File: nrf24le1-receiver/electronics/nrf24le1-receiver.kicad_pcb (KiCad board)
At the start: 2 copper layers, 19 x 25 mm, 20 parts, among them K1 CONN_3, K2 CONN_3, K3 CONN_3, K4 CONN_3, P1 CONN_1, P2 CONN_1, P3 CONN_1, SW1 BIND, U1 MCP1703, U2 NRF24LE1-MODULE-15X21

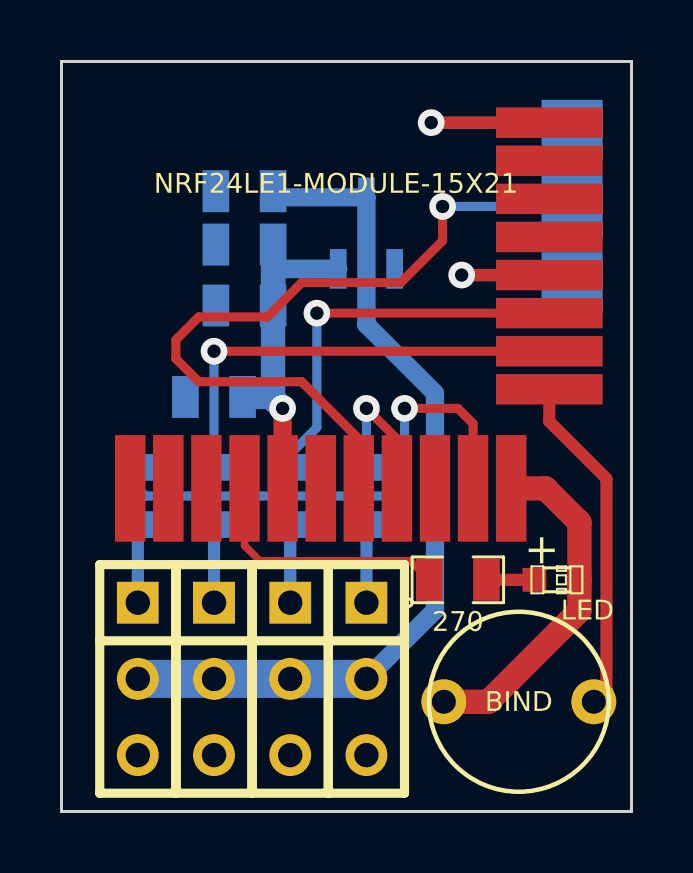
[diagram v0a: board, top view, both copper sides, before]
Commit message: Add Gerber for revision 2 PCB
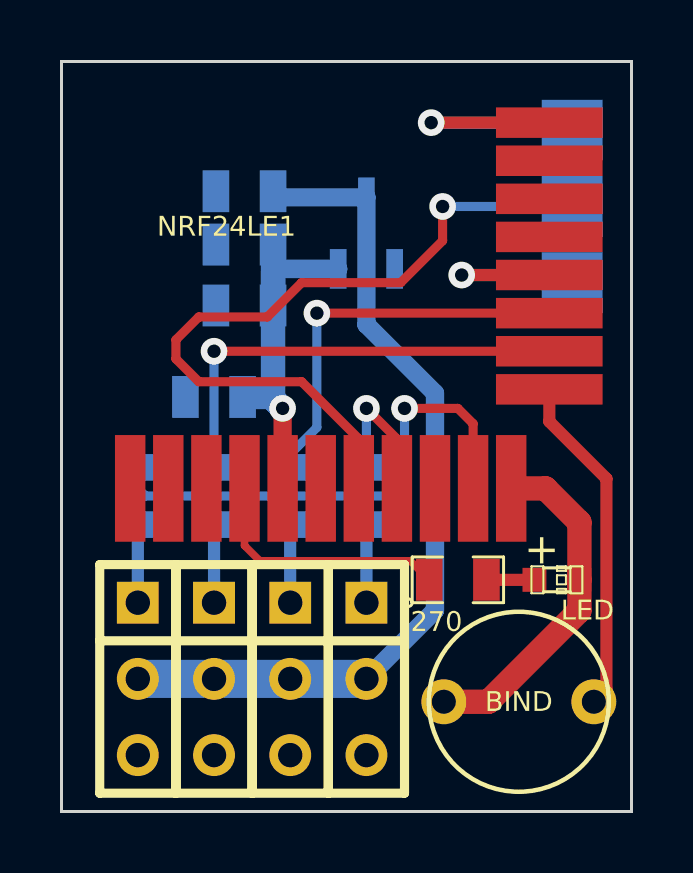
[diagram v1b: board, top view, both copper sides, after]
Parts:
- U2: value NRF24LE1-MODULE-15X21 -> NRF24LE1
